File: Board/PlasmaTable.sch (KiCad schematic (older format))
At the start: 48 parts, among them P1 CONN_20X2, P10 CONN_1, P11 CONN_1, P2 CONN_5, P3 CONN_5, P4 CONN_5, P5 CONN_5, P6 CONN_5, P7 CONN_5, P8 CONN_1, P9 CONN_1, Q1 TIP120, Q2 TIP120, Q3 TIP120, U1 7805, U2 7805, U3 7805, U4 7805

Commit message: Fixed errors made in first revision and plotted
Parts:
- Q1, Q2, Q3: footprint discret:TO220 -> PlasmaTable:TO220
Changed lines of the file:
@@
 F 0 "Q1" H 5250 6450 40  0000 R CNN
 F 1 "TIP120" H 5300 6750 40  0000 R CNN
-F 2 "discret:TO220" H 5180 6705 29  0001 C CNN
+F 2 "PlasmaTable:TO220" H 5180 6705 29  0001 C CNN
 F 3 "" H 5300 6600 60  0000 C CNN
 	1    5300 6600
@@
 F 0 "Q2" H 5850 6450 40  0000 R CNN
 F 1 "TIP120" H 5900 6750 40  0000 R CNN
-F 2 "discret:TO220" H 5780 6705 29  0001 C CNN
+F 2 "PlasmaTable:TO220" H 5780 6705 29  0001 C CNN
 F 3 "" H 5900 6600 60  0000 C CNN
 	1    5900 6600
@@
 F 0 "Q3" H 6450 6450 40  0000 R CNN
 F 1 "TIP120" H 6500 6750 40  0000 R CNN
-F 2 "discret:TO220" H 6380 6705 29  0001 C CNN
+F 2 "PlasmaTable:TO220" H 6380 6705 29  0001 C CNN
 F 3 "" H 6500 6600 60  0000 C CNN
 	1    6500 6600

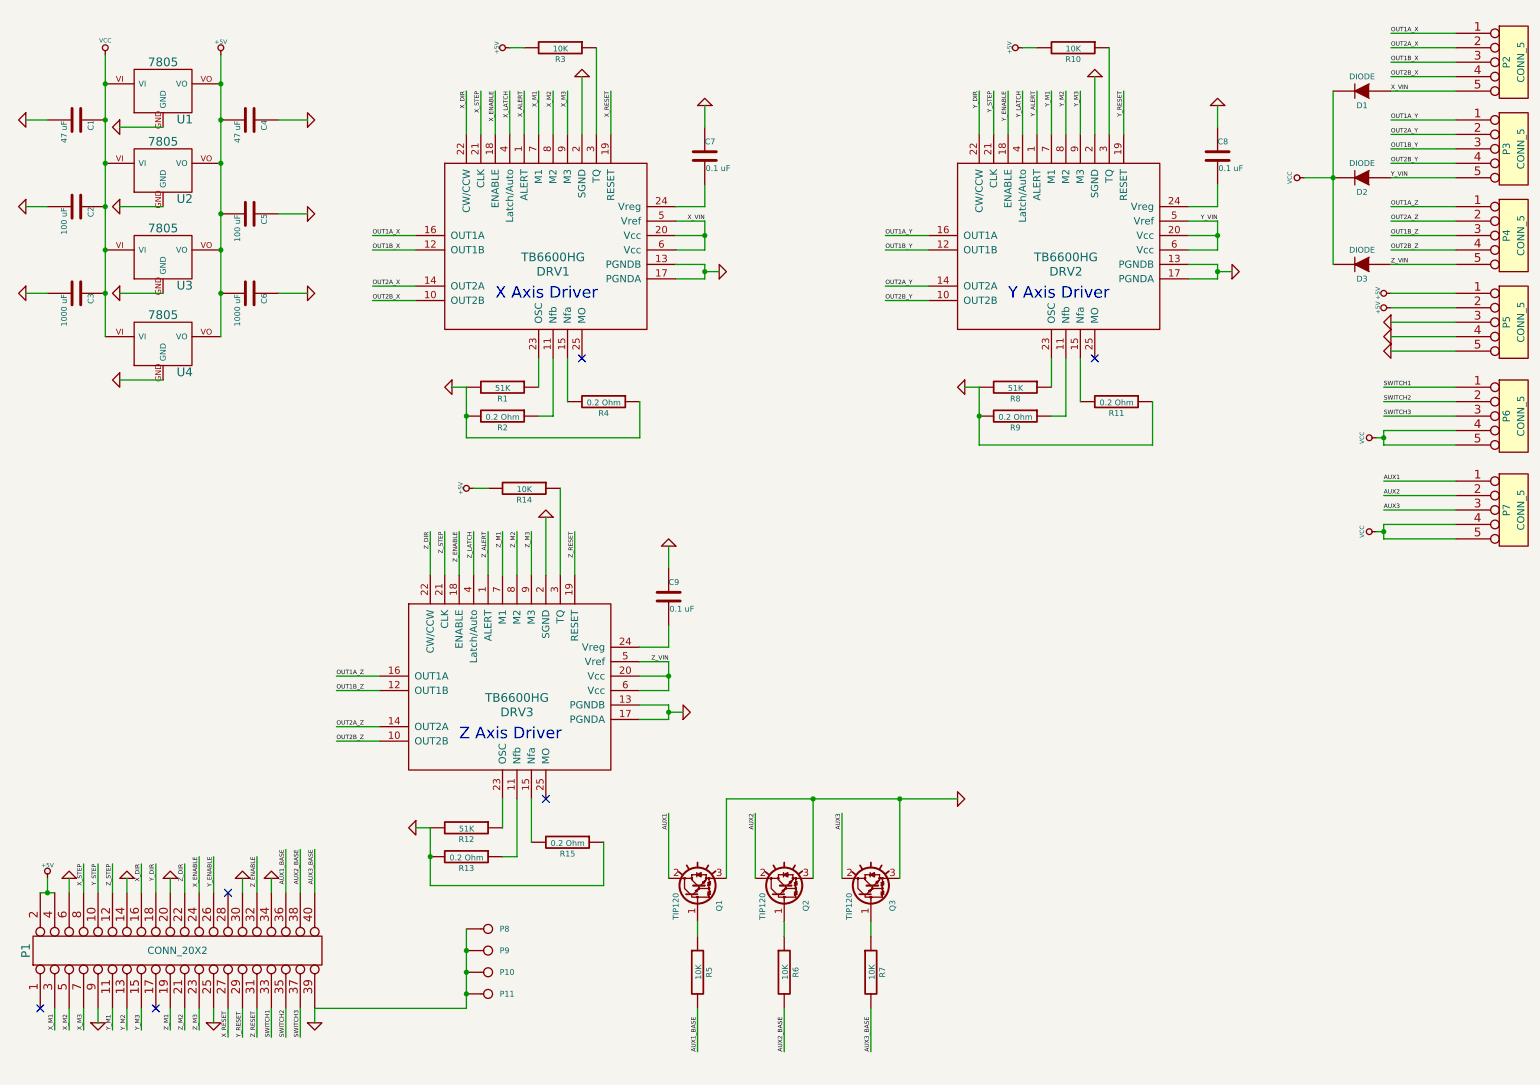
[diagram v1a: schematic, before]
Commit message: Updated shematic to hopefully protect from hf
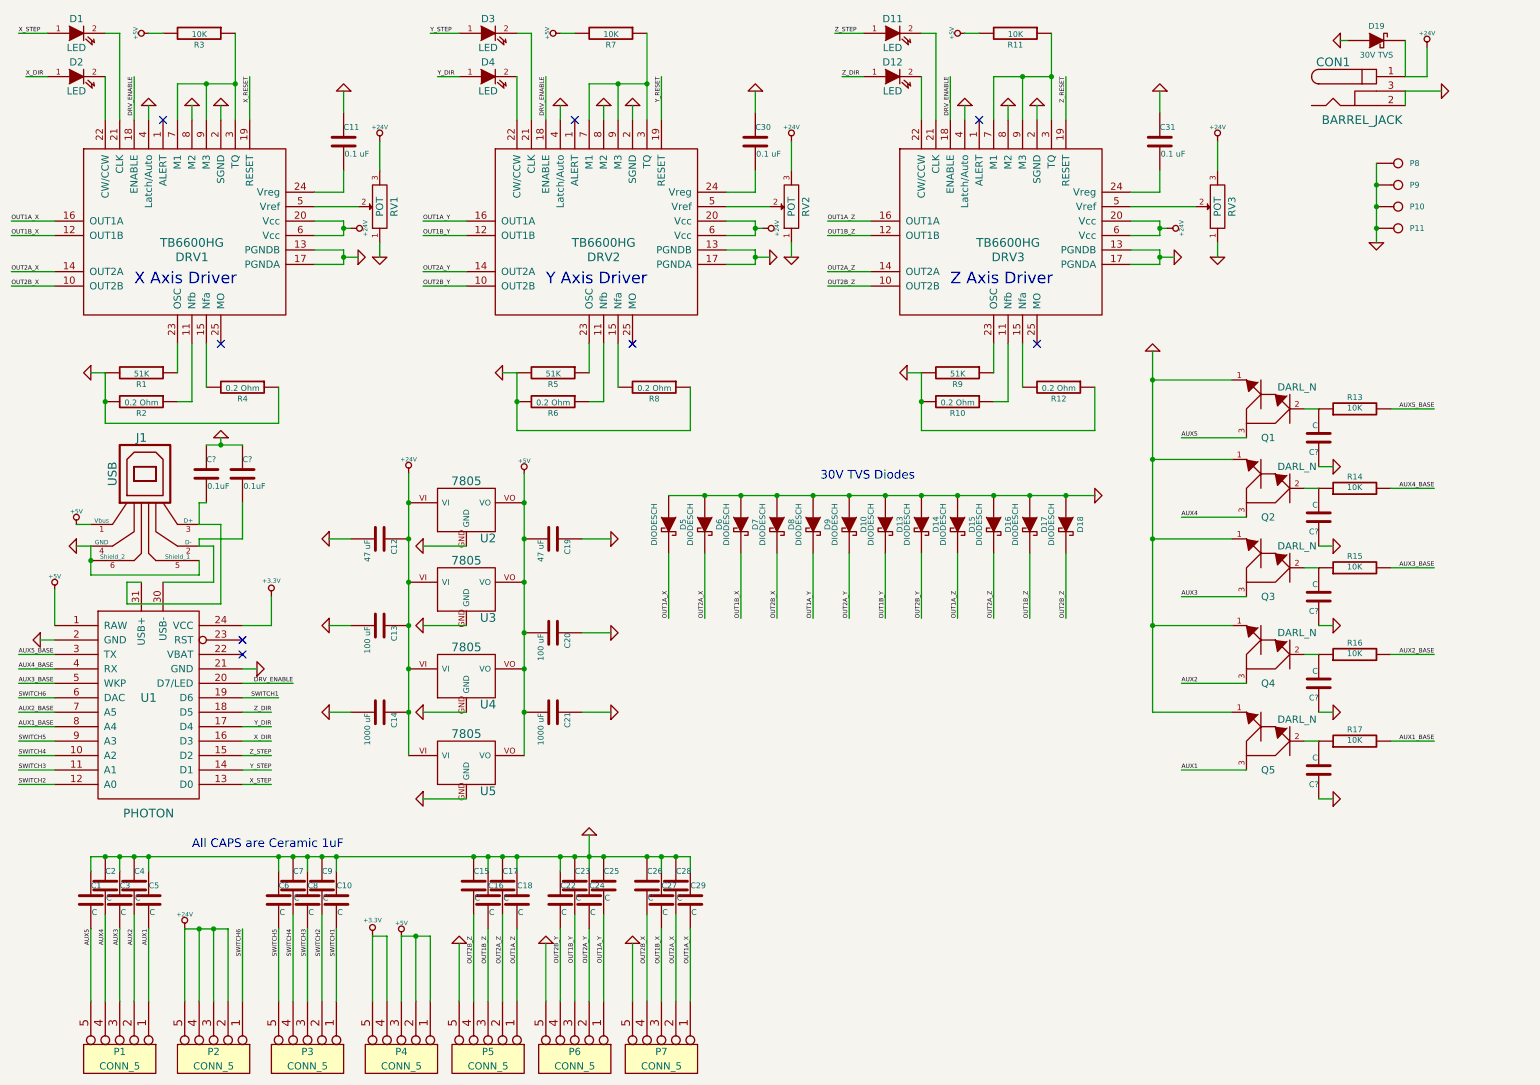
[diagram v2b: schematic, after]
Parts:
- removed D1, D2, D3: DIODE, discret:D3, symbol DIODE
- removed P1: CONN_20X2, pin_array:PIN_ARRAY_20X2, symbol CONN_20X2
- removed Q1, Q2, Q3: TIP120, PlasmaTable:TO220, symbol TIP120
- added C1, C10, C15, C16, C17, C18, C2, C22, C23, C24, C25, C26, C27, C28, C29, C3, C4, C5, C6, C7, C8, C9, C? (x5): C, symbol C
- added C? (x2): 0.1uF, symbol C
- added CON1: BARREL_JACK, symbol BARREL_JACK
- added D1, D11, D12, D2, D3, D4: LED, symbol LED
- added D10, D13, D14, D15, D16, D17, D18, D5, D6, D7, D8, D9: DIODESCH, symbol DIODESCH
- added D19: 30V TVS, symbol DIODESCH
- added J1: USB, symbol USB
- added P2: CONN_5, connect:SIL-5, symbol CONN_5
- added Q1, Q2, Q3, Q4, Q5: DARL_N, symbol DARL_N
- added R13, R14: 10K, discret:R3, symbol R
- added RV1, RV2, RV3: POT, symbol POT
- added U1: PHOTON, symbol PHOTON
- renumbered C7 to C11, C1 to C12, C2 to C13, C3 to C14, C4 to C19, C5 to C20, C6 to C21, C8 to C30, C9 to C31, P7 to P1, P6 to P3, P5 to P4, P4 to P5, P3 to P6, P2 to P7, R13 to R10, R14 to R11, R15 to R12, R7 to R15, R6 to R16, R5 to R17, R8 to R5, R9 to R6, R10 to R7, R11 to R8, R12 to R9, U1 to U2, U2 to U3, U3 to U4, U4 to U5
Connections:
- net X_LATCH is gone; now on net GND: DRV1.4 (Latch/Auto)
- net X_M1 is gone; now on an unnamed net: DRV1.7 (M1)
- net X_M2 is gone; now on net GND: DRV1.8 (M2)
- net X_M3 is gone; now on an unnamed net: DRV1.9 (M3)
- net Y_ENABLE is gone; now on net DRV_ENABLE: DRV2.18 (ENABLE)
- net Y_LATCH is gone; now on net GND: DRV2.4 (Latch/Auto)
- net Y_M1 is gone; now on an unnamed net: DRV2.7 (M1)
- net Y_M2 is gone; now on net GND: DRV2.8 (M2)
- net Y_M3 is gone; now on an unnamed net: DRV2.9 (M3)
- net Z_ENABLE is gone; now on net DRV_ENABLE: DRV3.18 (ENABLE)
- net Z_LATCH is gone; now on net GND: DRV3.4 (Latch/Auto)
- net Z_M1 is gone; now on an unnamed net: DRV3.7 (M1)
- net Z_M2 is gone; now on net GND: DRV3.8 (M2)
- net Z_M3 is gone; now on an unnamed net: DRV3.9 (M3)
- net +5V: now also P4.3, J1.1 (Vbus), U1.1 (RAW)
- net AUX1: now also C5.2, Q5.3
- net AUX1_BASE: now also U1.8 (A4)
- net AUX2: now also C4.2, Q4.3
- net AUX2_BASE: now also U1.7 (A5)
- net AUX3: now also C3.2, Q3.3
- net AUX3_BASE: now also U1.5 (WKP)
- net GND: now also P5.5, P6.5, P7.5, C1.1, C10.1, C15.1, C16.1, C17.1, C18.1, C2.1, C22.1, C23.1, C24.1, C25.1, C26.1, C27.1, C28.1, C29.1, C3.1, C4.1, C5.1, C6.1, C7.1, C8.1, C9.1, C?.1, C?.1, C?.1, C?.1, C?.1, C?.1, C?.1, CON1.2, CON1.3, D10.1 (A), D13.1 (A), D14.1 (A), D15.1 (A), D16.1 (A), D17.1 (A), D18.1 (A), D19.1 (A), D5.1 (A), D6.1 (A), D7.1 (A), D8.1 (A), D9.1 (A), J1.4 (GND), J1.5 (Shield_1), J1.6 (Shield_2), Q1.1, Q2.1, Q3.1, Q4.1, Q5.1, RV1.1, RV2.1, RV3.1, U1.2 (GND), U1.21 (GND); no longer P4.3, P4.4, P4.5
- net OUT1A_X: now also C29.2, D5.2 (K)
- net OUT1A_Y: now also C25.2, D9.2 (K)
- net OUT1A_Z: now also C18.2, D15.2 (K)
- net OUT1B_X: now also C27.2, D7.2 (K)
- net OUT1B_Y: now also C23.2, D13.2 (K)
- net OUT1B_Z: now also C16.2, D17.2 (K)
- net OUT2A_X: now also C28.2, D6.2 (K)
- net OUT2A_Y: now also C24.2, D10.2 (K)
- net OUT2A_Z: now also C17.2, D16.2 (K)
- net OUT2B_X: now also C26.2, D8.2 (K)
- net OUT2B_Y: now also C22.2, D14.2 (K)
- net OUT2B_Z: now also C15.2, D18.2 (K)
- net SWITCH1: now also C10.2, U1.19 (D6)
- net SWITCH2: now also C9.2, U1.12 (A0)
- net SWITCH3: now also C8.2, U1.11 (A1)
- net X_DIR: now also D2.1 (A), U1.16 (D3); no longer DRV1.22 (CW/CCW)
- net X_STEP: now also D1.1 (A), U1.13 (D0); no longer DRV1.21 (CLK)
- net Y_DIR: now also D4.1 (A), U1.17 (D4); no longer DRV2.22 (CW/CCW)
- net Y_STEP: now also D3.1 (A), U1.14 (D1); no longer DRV2.21 (CLK)
- net Z_DIR: now also D12.1 (A), U1.18 (D5); no longer DRV3.22 (CW/CCW)
- net Z_STEP: now also D11.1 (A), U1.15 (D2); no longer DRV3.21 (CLK)
- net at R17.1: now also C?.2, Q5.2
- net at R16.1: now also C?.2, Q4.2
- net at R15.1: now also C?.2, Q3.2
- net VCC renamed +24V
- net +24V: now also DRV1.20 (Vcc), DRV1.6 (Vcc), DRV2.20 (Vcc), DRV2.6 (Vcc), DRV3.20 (Vcc), DRV3.6 (Vcc), CON1.1, D19.2 (K), P2.2, P2.3, P2.4, P2.5, RV1.3, RV2.3, RV3.3; no longer P1.4, P1.5, P3.4, P3.5
- net X_ALERT: no longer names the net of DRV1.1 (ALERT)
- net X_ENABLE renamed DRV_ENABLE
- net DRV_ENABLE: now also U1.20 (D7/LED)
- removed net X_VIN: DRV1.20 (Vcc), DRV1.5 (Vref), DRV1.6 (Vcc), P7.5
- net Y_ALERT: no longer names the net of DRV2.1 (ALERT)
- removed net Y_VIN: DRV2.20 (Vcc), DRV2.5 (Vref), DRV2.6 (Vcc), P6.5
- net Z_ALERT: no longer names the net of DRV3.1 (ALERT)
- removed net Z_VIN: DRV3.20 (Vcc), DRV3.5 (Vref), DRV3.6 (Vcc), P5.5
- new net: D1.2 (K), DRV1.21 (CLK)
- new net: D2.2 (K), DRV1.22 (CW/CCW)
- new net: DRV1.5 (Vref), RV1.2
- new net: D3.2 (K), DRV2.21 (CLK)
- new net: D4.2 (K), DRV2.22 (CW/CCW)
- new net: DRV2.5 (Vref), RV2.2
- new net: D11.2 (K), DRV3.21 (CLK)
- new net: D12.2 (K), DRV3.22 (CW/CCW)
- new net: DRV3.5 (Vref), RV3.2
- new net: C?.2, Q2.2, R14.1
- new net: C?.2, Q1.2, R13.1
- new net: C?.2, J1.2 (D-), U1.30 (USB-)
- new net: C?.2, J1.3 (D+), U1.31 (USB+)
- new net +3.3V: P4.4, P4.5, U1.24 (VCC)
- new net AUX4: C2.2, P1.4, Q2.3
- new net AUX4_BASE: R14.2, U1.4 (RX)
- new net AUX5: C1.2, P1.5, Q1.3
- new net AUX5_BASE: R13.2, U1.3 (TX)
- new net SWITCH4: C7.2, P3.4, U1.10 (A2)
- new net SWITCH5: C6.2, P3.5, U1.9 (A3)
- new net SWITCH6: P2.1, U1.6 (DAC)
- no-connect marks 6 -> 8
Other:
- note added: "30V TVS Diodes"
- note added: "All CAPS are Ceramic 1uF"
- moved on the sheet: C11, C12, C13, C14, C19, C20, C21, C30, C31, DRV1, DRV2, DRV3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
